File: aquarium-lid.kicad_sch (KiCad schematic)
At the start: 29 parts, among them J2 Fan1, J3 Fan2, J4 Temp Sensor, J5 USB_C_Receptacle_USB2.0_14P, Q1 2N7002, Q2 2N7002, Q3 2N7002, SW1 Action 1, U1 ESP32-C3-WROOM-02

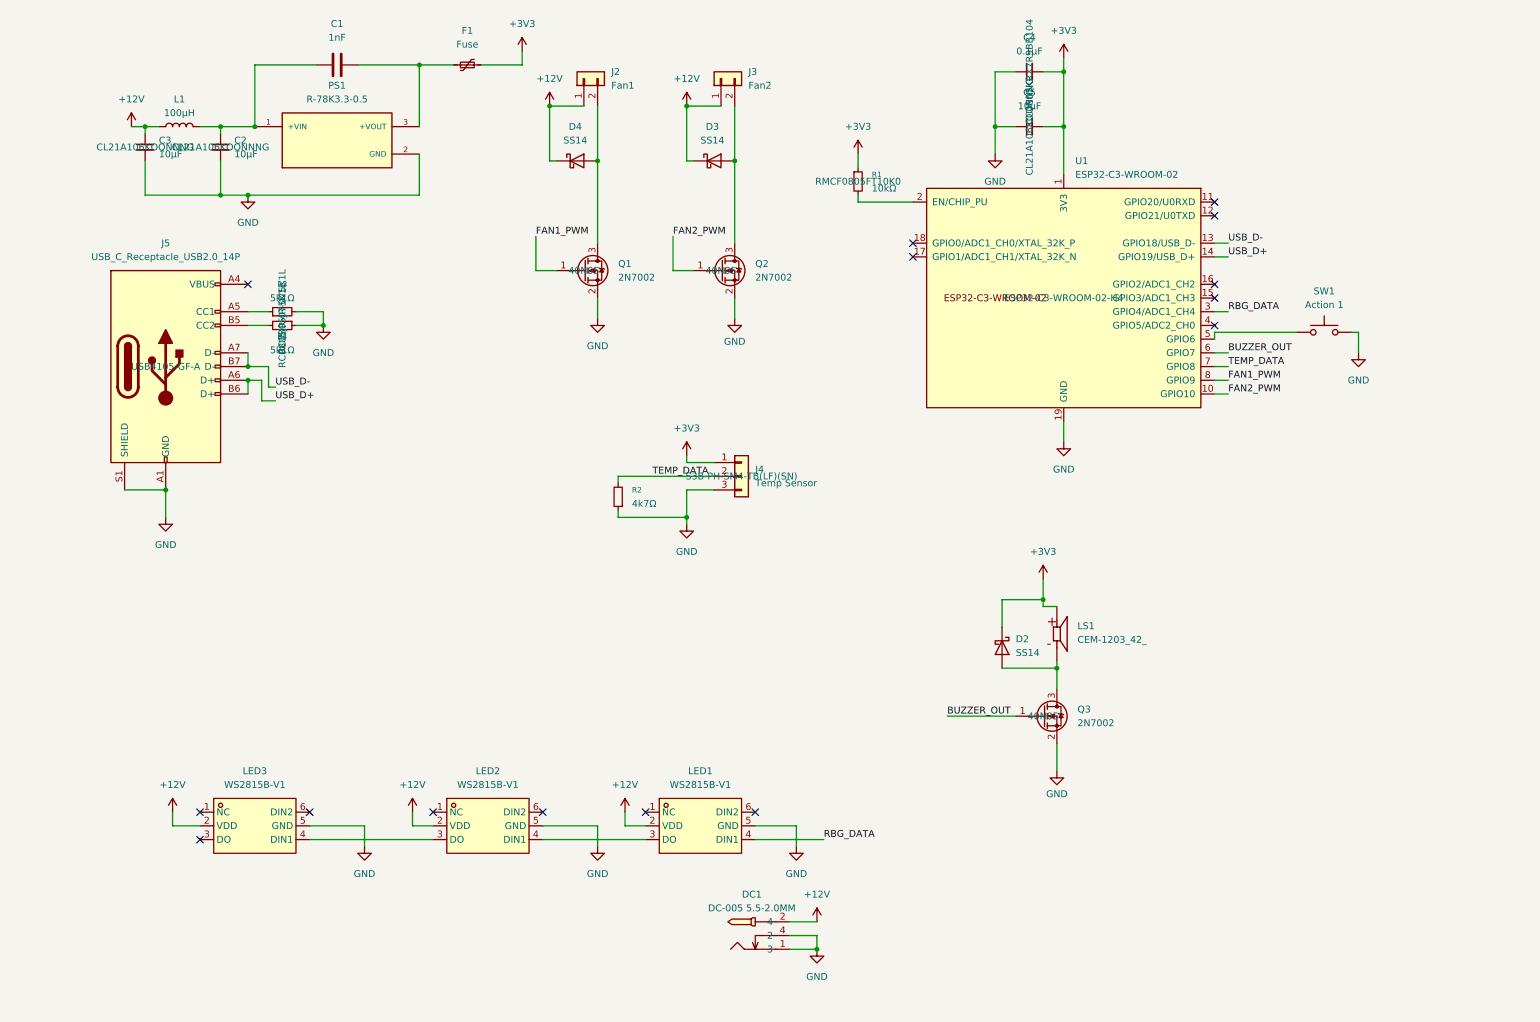
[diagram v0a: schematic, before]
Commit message: Quick save
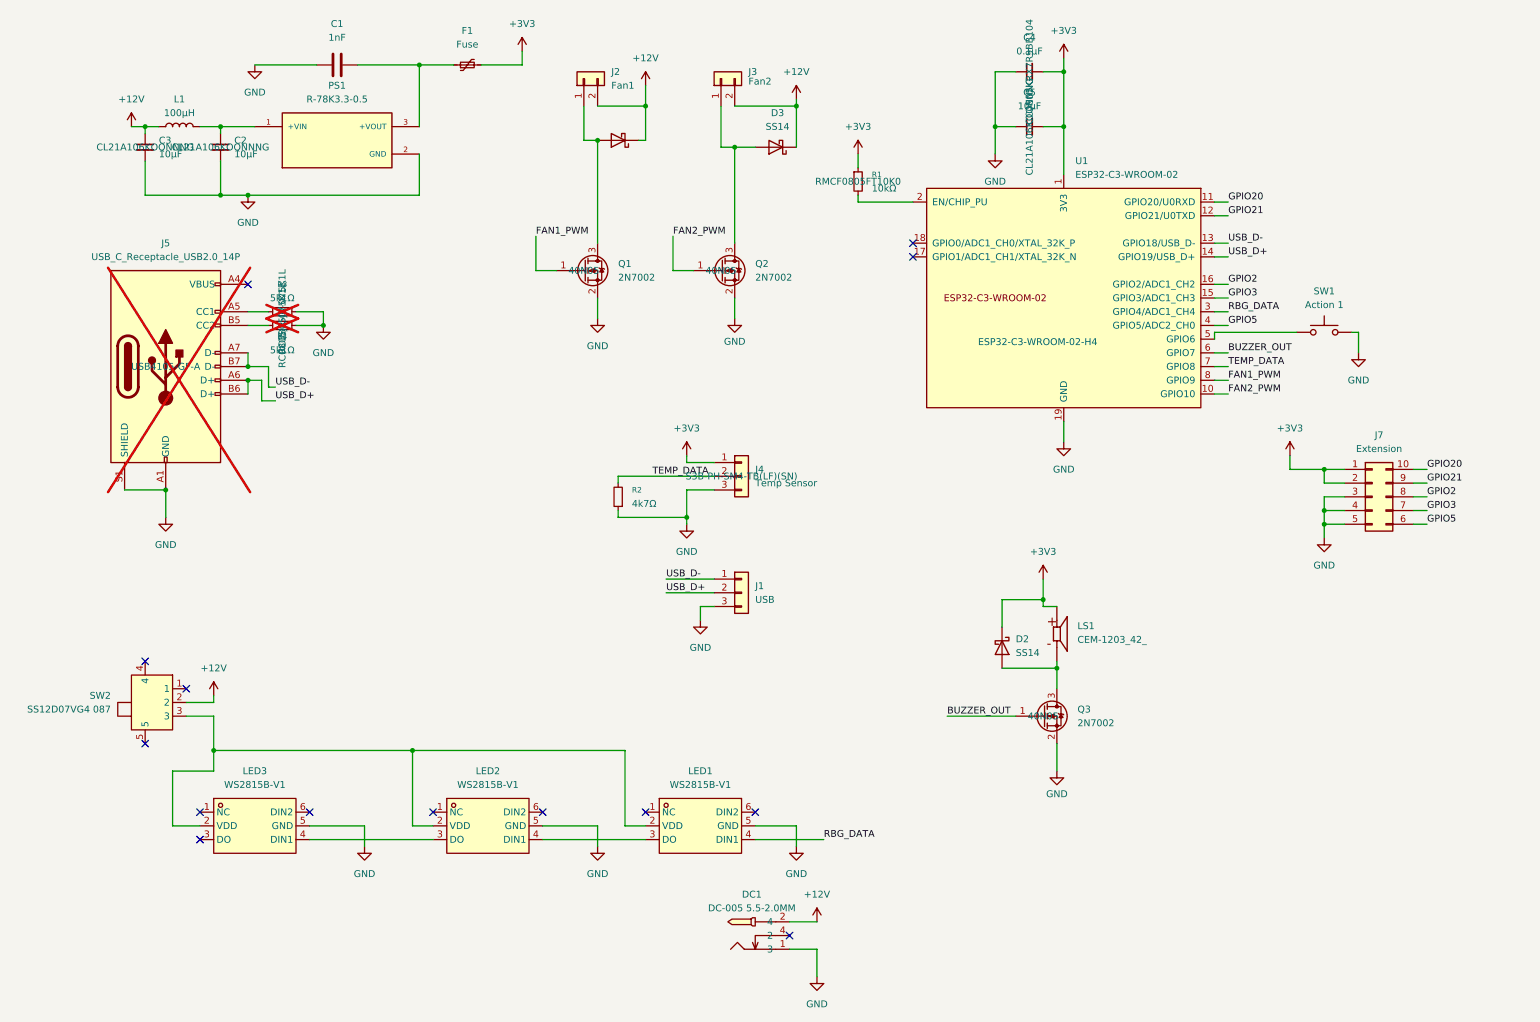
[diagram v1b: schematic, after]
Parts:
- added J1: USB, Connector_PinHeader_2.54mm:PinHeader_1x03_P2.54mm_Vertical, symbol Connector_Generic:Conn_01x03
- added J7: Extension, Connector_PinHeader_2.54mm:PinHeader_2x05_P2.54mm_Vertical, symbol Connector_Generic:Conn_02x05_Counter_Clockwise
- added SW2: SS12D07VG4 087, easyeda2kicad:SW-TH_SS12D07VG4, symbol easyeda2kicad:SS12D07VG4087
- J5, R3, R4: now not fitted
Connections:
- net +12V: now also J2.2 (Pin_2), J3.2 (Pin_2), SW2.2; no longer J2.1 (Pin_1), J3.1 (Pin_1), LED1.2 (VDD), LED2.2 (VDD), LED3.2 (VDD)
- net +3V3: now also J7.1 (Pin_1), J7.2 (Pin_2)
- net GND: now also C1.1, J1.3 (Pin_3), J7.3 (Pin_3), J7.4 (Pin_4), J7.5 (Pin_5); no longer DC1.4 (2)
- net USB_D+: now also J1.2 (Pin_2)
- net USB_D-: now also J1.1 (Pin_1)
- net at D3.2 (A), Q2.3 (D): now also J3.1 (Pin_1); no longer J3.2 (Pin_2)
- net at C2.1, L1.2, PS1.1 (+VIN): no longer C1.1
- net GPIO20: now reaches U1.11 (GPIO20/U0RXD)
- net GPIO20: now also J7.10 (Pin_10)
- net GPIO21: now reaches U1.12 (GPIO21/U0TXD)
- net GPIO21: now also J7.9 (Pin_9)
- net GPIO3: now reaches U1.15 (GPIO3/ADC1_CH3)
- net GPIO3: now also J7.7 (Pin_7)
- net GPIO2: now reaches U1.16 (GPIO2/ADC1_CH2)
- net GPIO2: now also J7.8 (Pin_8)
- net GPIO5: now reaches U1.4 (GPIO5/ADC2_CH0)
- net GPIO5: now also J7.6 (Pin_6)
- net at D4.2 (A), Q1.3 (D): now also J2.1 (Pin_1); no longer J2.2 (Pin_2)
- new net: LED1.2 (VDD), LED2.2 (VDD), LED3.2 (VDD), SW2.3
- no-connect marks 15 -> 14
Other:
- moved on the sheet: D3

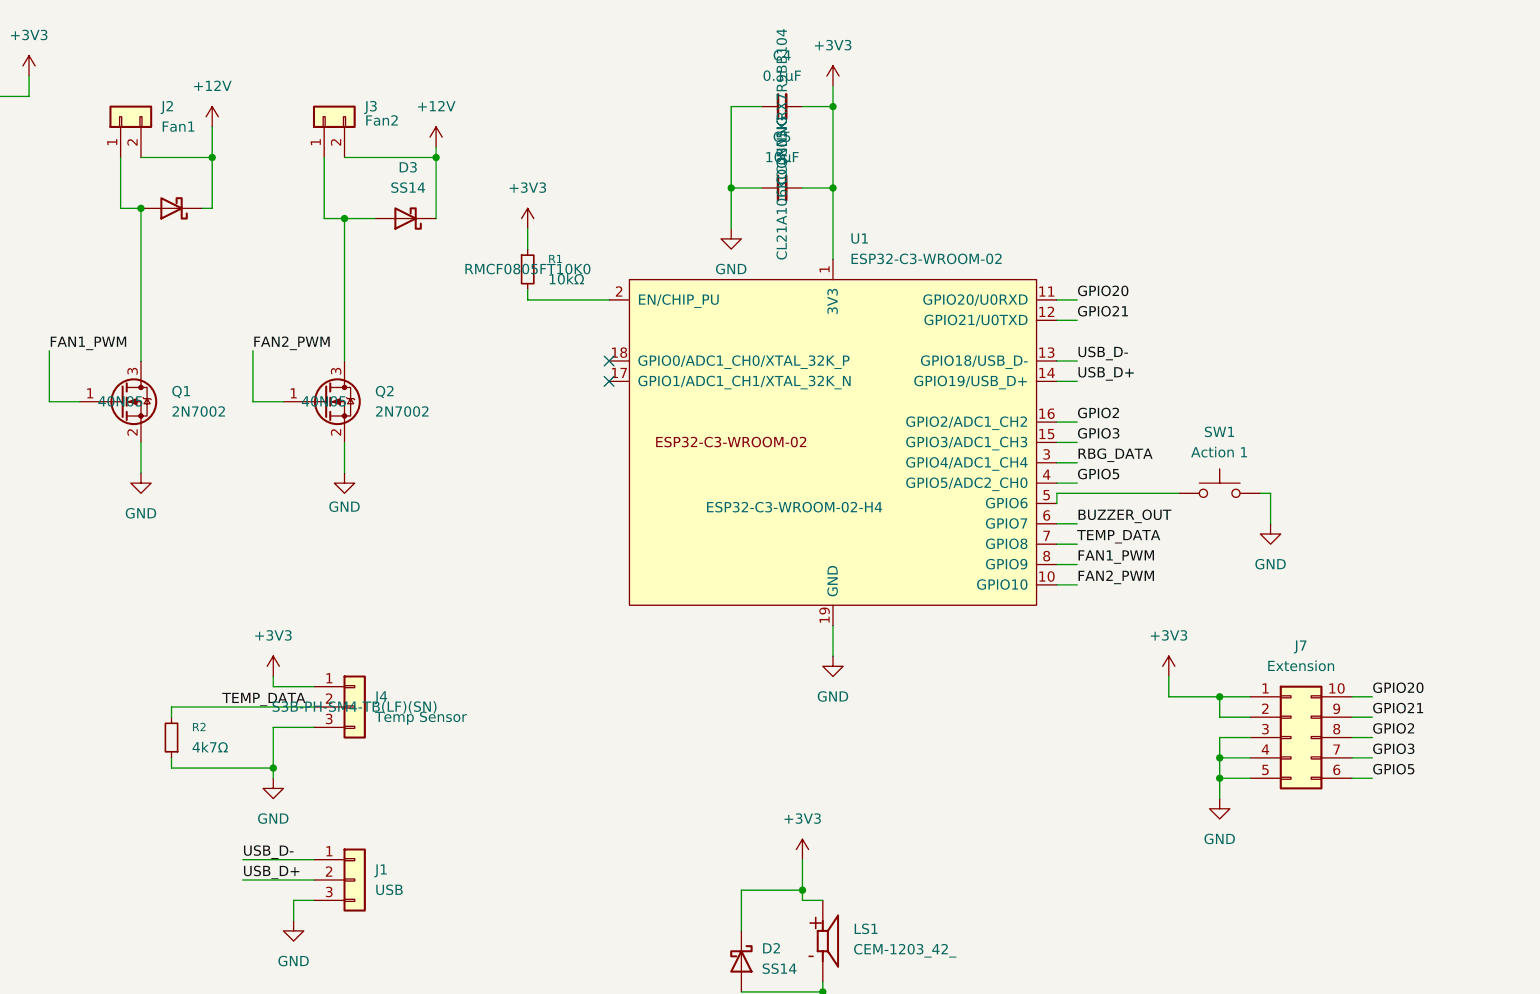
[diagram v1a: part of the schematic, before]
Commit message: New PCB
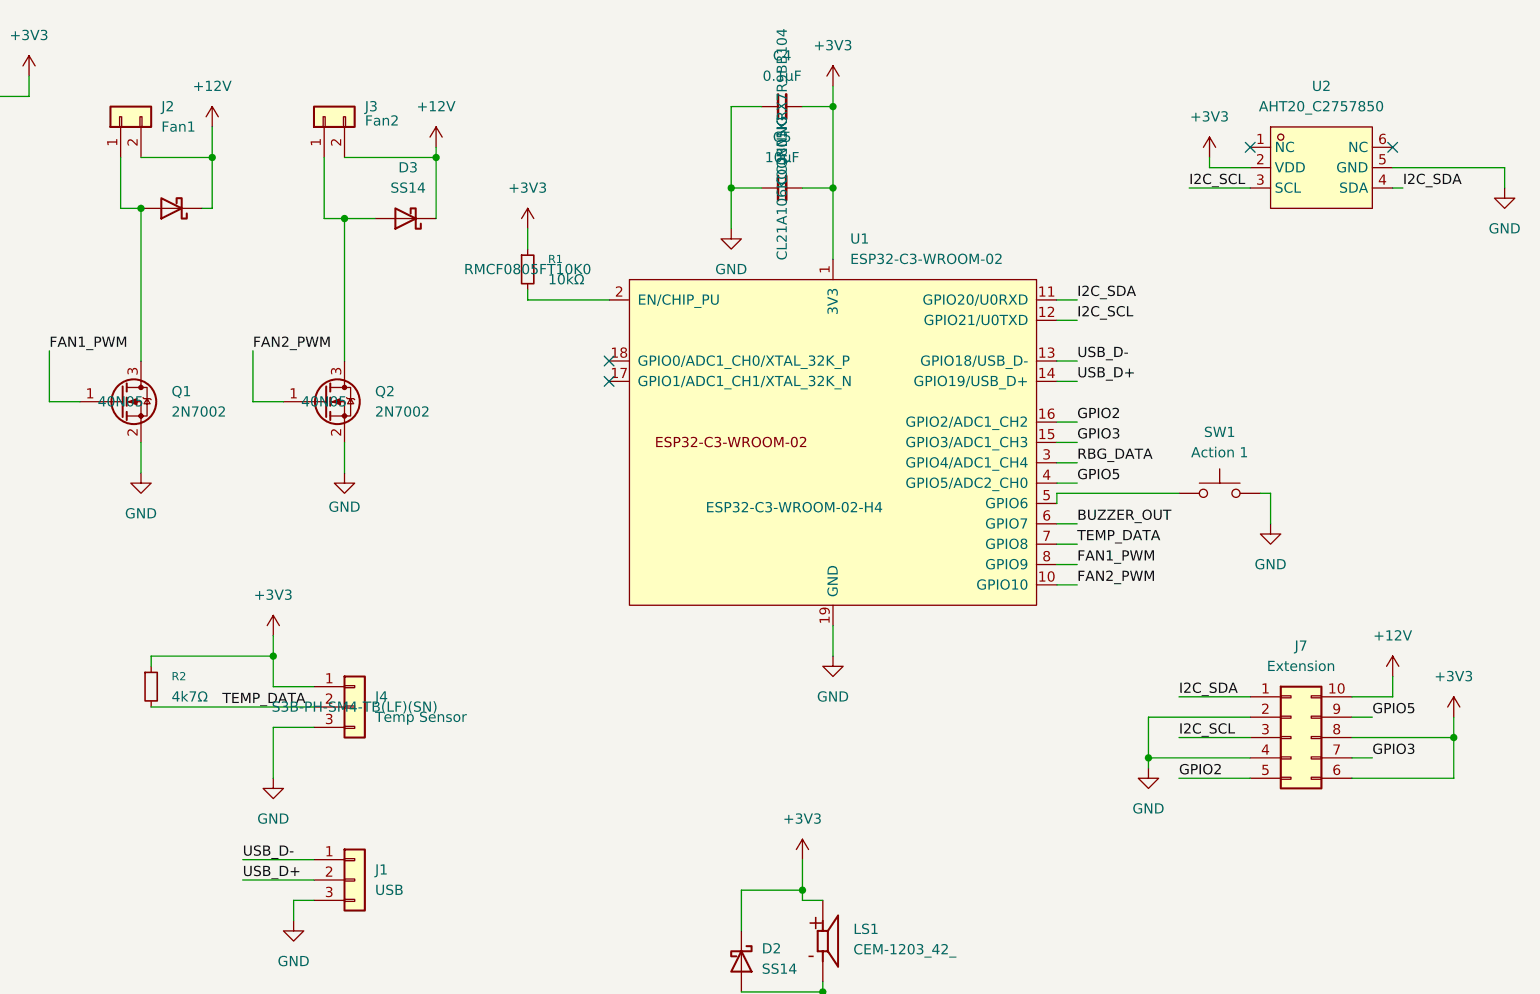
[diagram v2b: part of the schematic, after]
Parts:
- added U2: AHT20_C2757850, easyeda2kicad:SENSOR-SMD_L3.0-W3.0-P1.00-BR, symbol easyeda2kicad:AHT20_C2757850
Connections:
- net +12V: now also J7.10 (Pin_10)
- net +3V3: now also J7.6 (Pin_6), J7.8 (Pin_8), R2.1, U2.2 (VDD); no longer J7.1 (Pin_1), J7.2 (Pin_2)
- net GND: now also J7.2 (Pin_2), U2.5 (GND); no longer J7.3 (Pin_3), J7.5 (Pin_5), R2.1
- net GPIO2: now also J7.5 (Pin_5); no longer J7.8 (Pin_8)
- net GPIO5: now also J7.9 (Pin_9); no longer J7.6 (Pin_6)
- net GPIO20 renamed I2C_SDA
- net I2C_SDA: now also J7.1 (Pin_1), U2.4 (SDA); no longer J7.10 (Pin_10)
- net GPIO21 renamed I2C_SCL
- net I2C_SCL: now also J7.3 (Pin_3), U2.3 (SCL); no longer J7.9 (Pin_9)
- no-connect marks 14 -> 16
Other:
- moved on the sheet: R2

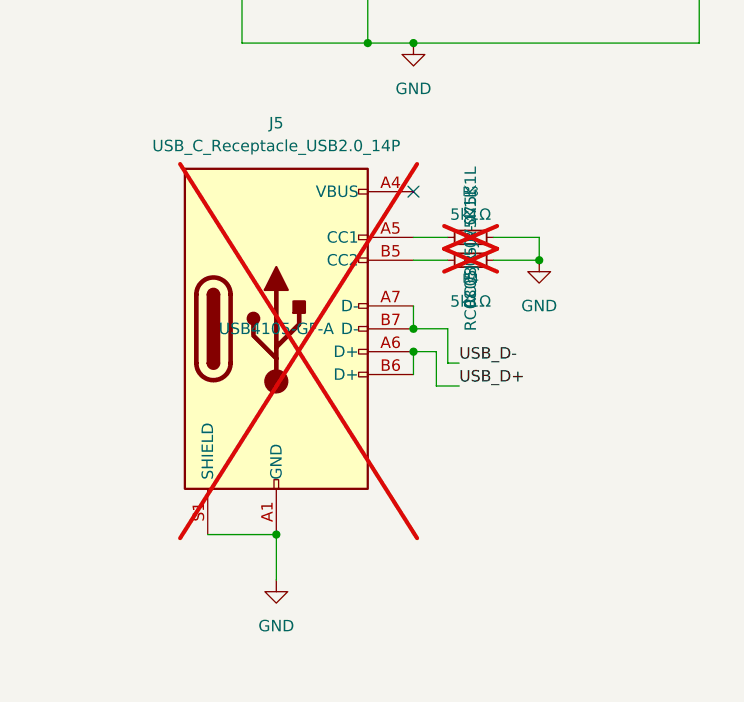
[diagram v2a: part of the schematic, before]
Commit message: Changes
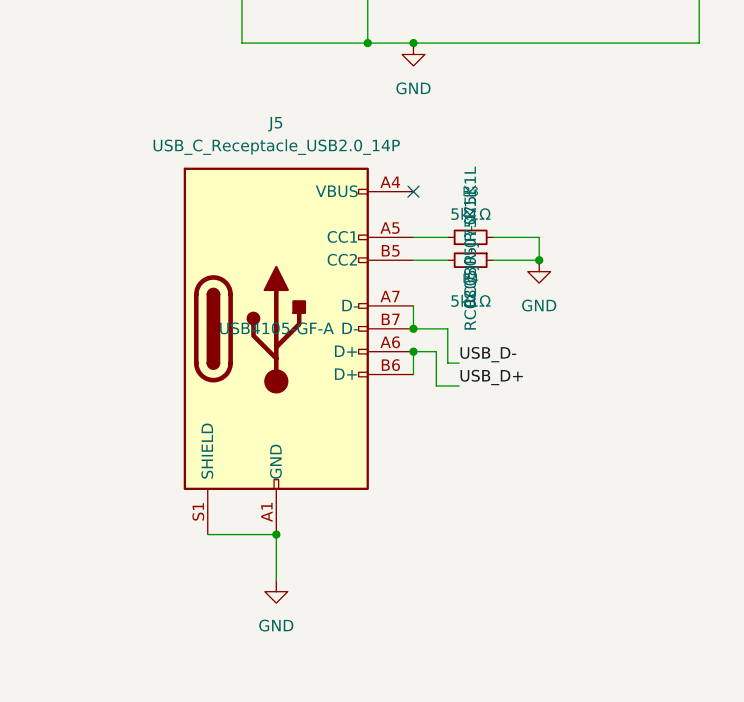
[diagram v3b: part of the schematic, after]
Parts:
- J5, R3, R4: now fitted
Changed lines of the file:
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@@
 		(in_bom yes)
 		(on_board yes)
-		(dnp yes)
+		(dnp no)
 		(property "Reference" "R4"
 			(at 50.8 73.152 90)
@@
 		(in_bom yes)
 		(on_board yes)
-		(dnp yes)
+		(dnp no)
 		(fields_autoplaced yes)
 		(property "Reference" "J5"
@@
 		(in_bom yes)
 		(on_board yes)
-		(dnp yes)
+		(dnp no)
 		(property "Reference" "R3"
 			(at 50.8 63.5 90)
